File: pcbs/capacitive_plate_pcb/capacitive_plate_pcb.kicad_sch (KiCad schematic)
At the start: 38 parts, among them J1 BM09B-SRSS-TB_LF__SN_, J2 SM08B-SRSS-TB_LF__SN_, U1 ATMXT336UD-MAUHA1, U2 ICM-42670-P, U3 MCP1824T-3302E_OT

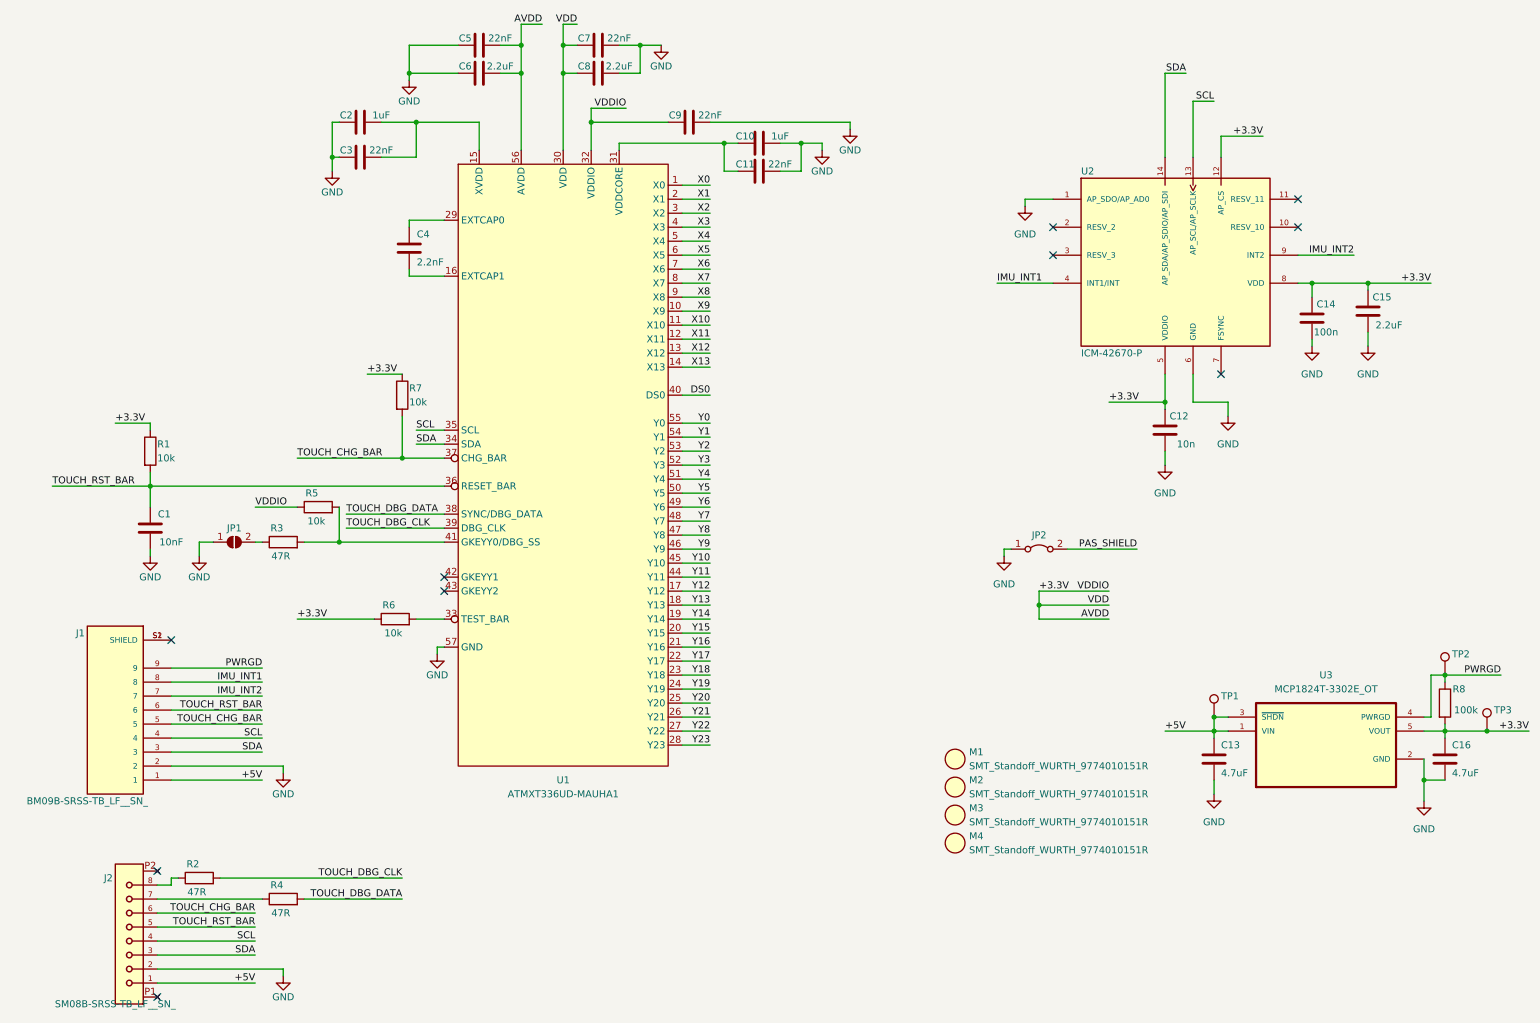
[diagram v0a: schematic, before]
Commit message: R01 plate pcb
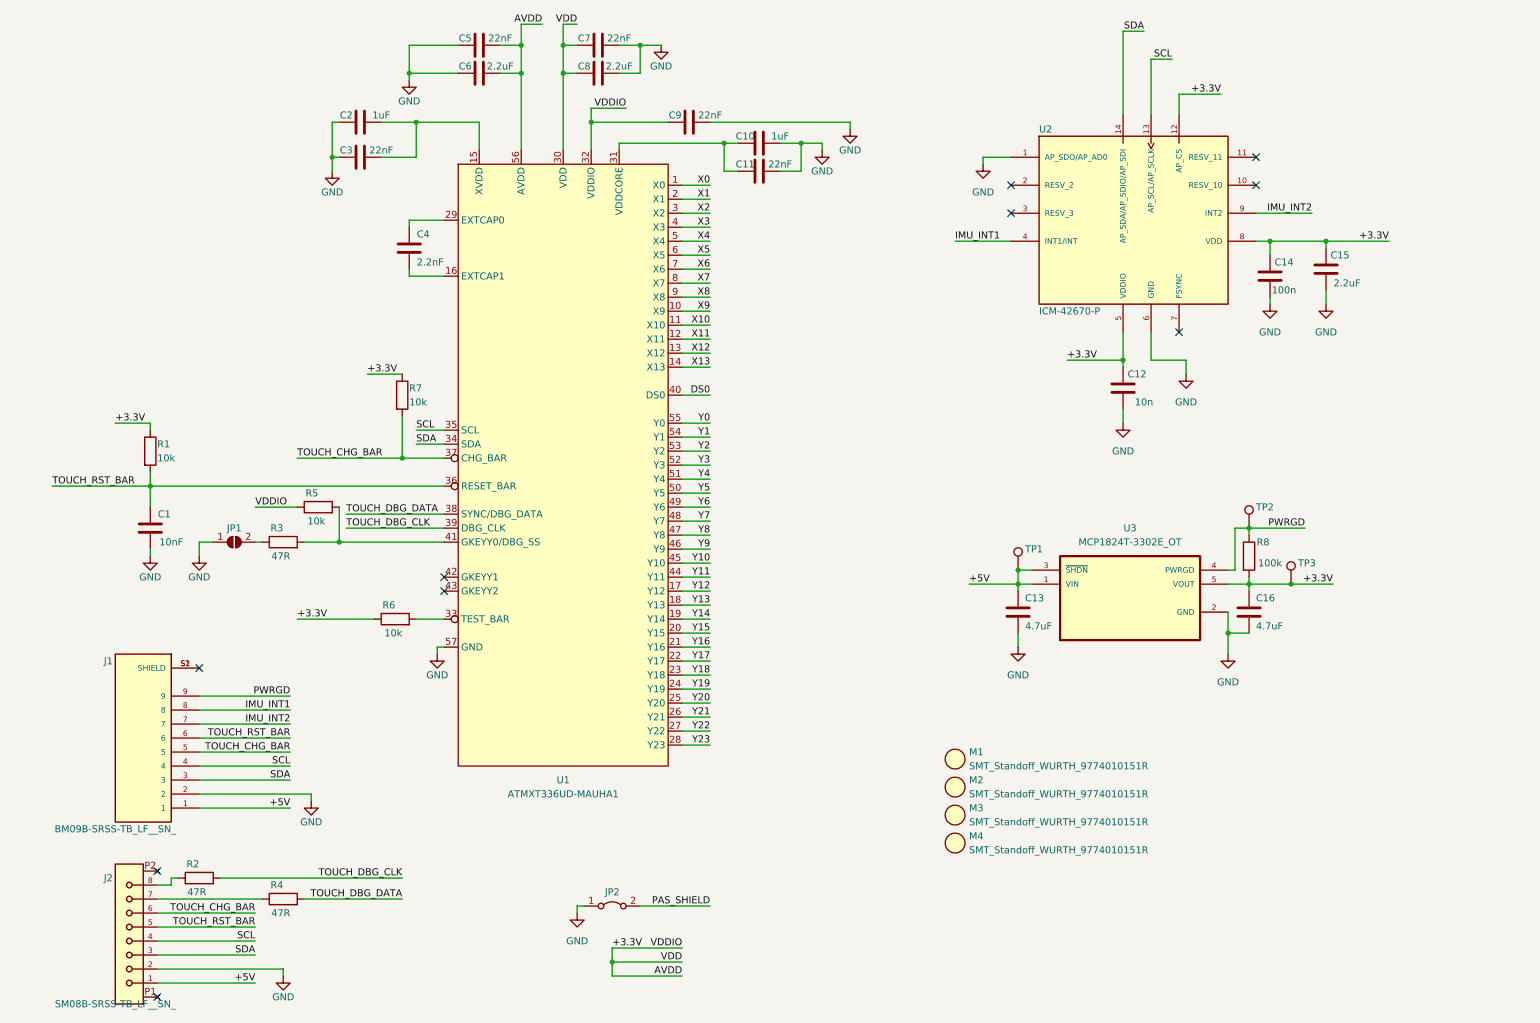
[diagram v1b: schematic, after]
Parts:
- J1: Availability In Stock -> (none); Check_prices https://www.snapeda.com/parts/BM09B-SRSS-TB(LF)(SN)/JST+Sal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 -> (none); MANUFACTURER JST Sales America Inc. -> (none); MAXIMUM_PACKAGE_HEIGHT 6.3 mm -> (none); MF JST Sales -> (none); MP BM09B-SRSS-TB(LF)(SN) -> (none); Manufacturer (none) -> JST; Manufacturer number (none) -> BM09B-SRSS-TB(LF)(SN); PARTREV N/A -> (none); Package None -> (none); Price None -> (none); SNAPEDA_PN BM09B-SRSS-TB(LF)(SN) -> (none); STANDARD Manufacturer Recommendations -> (none); SnapEDA_Link https://www.snapeda.com/parts/BM09B-SRSS-TB(LF)(SN)/JST+Sal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 -> (none); Supplier (none) -> Farnell; Supplier code (none) -> 1679135; Supplier website (none) -> https://uk.farnell.com/jst-japan-solderless-terminals/bm09b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
- J2: Availability In Stock -> (none); Check_prices https://www.snapeda.com/parts/SM08B-SRSS-TB(LF)(SN)/JST+Sal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 -> (none); MANUFACTURER JST -> (none); MF JST Sales -> (none); MP SM08B-SRSS-TB(LF)(SN) -> (none); Manufacturer (none) -> JST; Manufacturer number (none) -> SM08B-SRSS-TB(LF)(SN); Package None -> (none); Price None -> (none); SnapEDA_Link https://www.snapeda.com/parts/SM08B-SRSS-TB(LF)(SN)/JST+Sal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 -> (none); Supplier (none) -> Farnell; Supplier code (none) -> 1679124; Supplier website (none) -> https://uk.farnell.com/jst-japan-solderless-terminals/sm08b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
- M1, M2, M3, M4: Manufacturer (none) -> Wurth electronik; Manufacturer number (none) -> 9774010151R; Supplier (none) -> Farnell; Supplier code (none) -> 2766287; Supplier website (none) -> https://uk.farnell.com/wurth-elektronik/9774010151r/standof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
- R5, R6, R7, R8: footprint Capacitor_SMD:C_0603_1608Metric -> Resistor_SMD:R_0603_1608Metric
- U1: Manufacturer (none) -> Microchip Technology; Manufacturer number (none) -> ATMXT336UD-MAUHA1; Supplier (none) -> DigiKey; Supplier code (none) -> 150-ATMXT336UD-MAUHA1-ND; Supplier website (none) -> https://www.digikey.co.uk/en/products/detail/microchip-tech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
- U2: Availability In Stock -> (none); Check_prices https://www.snapeda.com/parts/ICM-42670-P/TDK+InvenSense/vi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 -> (none); MF TDK InvenSense -> (none); MP ICM-42670-P -> (none); Manufacturer (none) -> TDK InvenSense; Manufacturer number (none) -> ICM-42670-P; Package None -> (none); Price None -> (none); Purchase-URL https://www.snapeda.com/api/url_track_click_mouser/?unipart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 -> (none); SnapEDA_Link https://www.snapeda.com/parts/ICM-42670-P/TDK+InvenSense/vi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 -> (none); Supplier (none) -> Mouser; Supplier code (none) -> 410-ICM-42670-P; Supplier website (none) -> https://www.mouser.co.uk/ProductDetail/TDK-InvenSense/ICM-4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
- U3: Availability In Stock -> (none); MF Microchip -> (none); MP MCP1824T-3302E/OT -> (none); Manufacturer (none) -> Microchip; Manufacturer number (none) -> MCP1824T-3302E/OT; Price None -> (none); Supplier (none) -> Mouser; Supplier code (none) -> 579-MCP1824T-3302EOT; Supplier website (none) -> https://www.mouser.co.uk/ProductDetail/Microchip-Technology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
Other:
- moved on the sheet: C12, C13, C14, C15, C16, J1, JP2, R8, TP1, TP2, TP3, U2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
